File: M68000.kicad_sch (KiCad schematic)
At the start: 50 parts, among them J1 JTAG1, J2 USB_B, SW1 Util_SW, SW2 RESET_SW, SW3 STEP_SW, U1 MAX699, U2 XC9572, U3 MC68000FN, X1 ECS-2200B-080

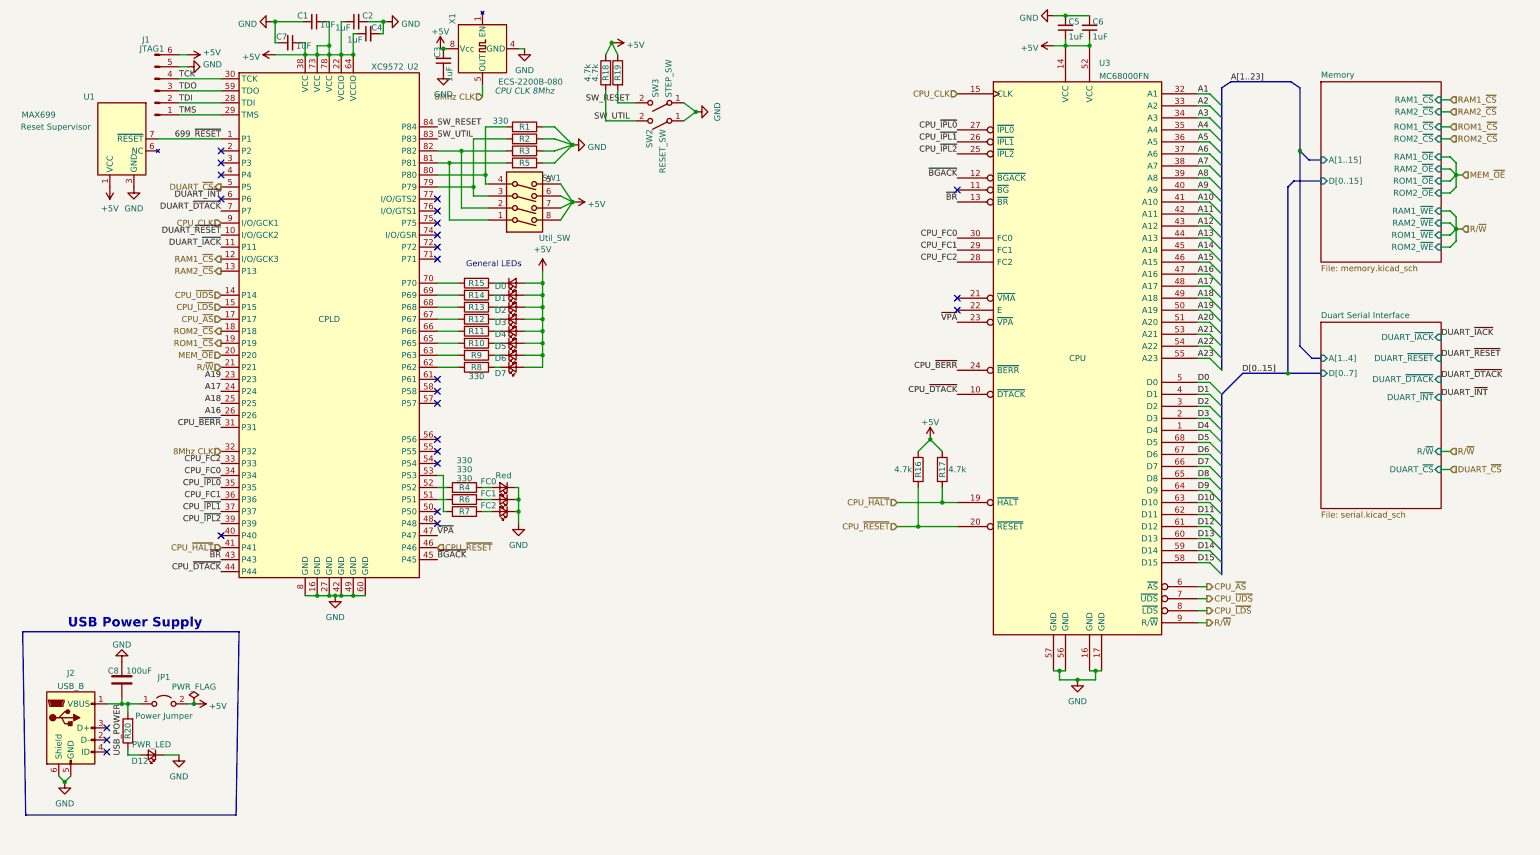
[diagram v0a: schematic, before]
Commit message: Submitted to JLCPCB
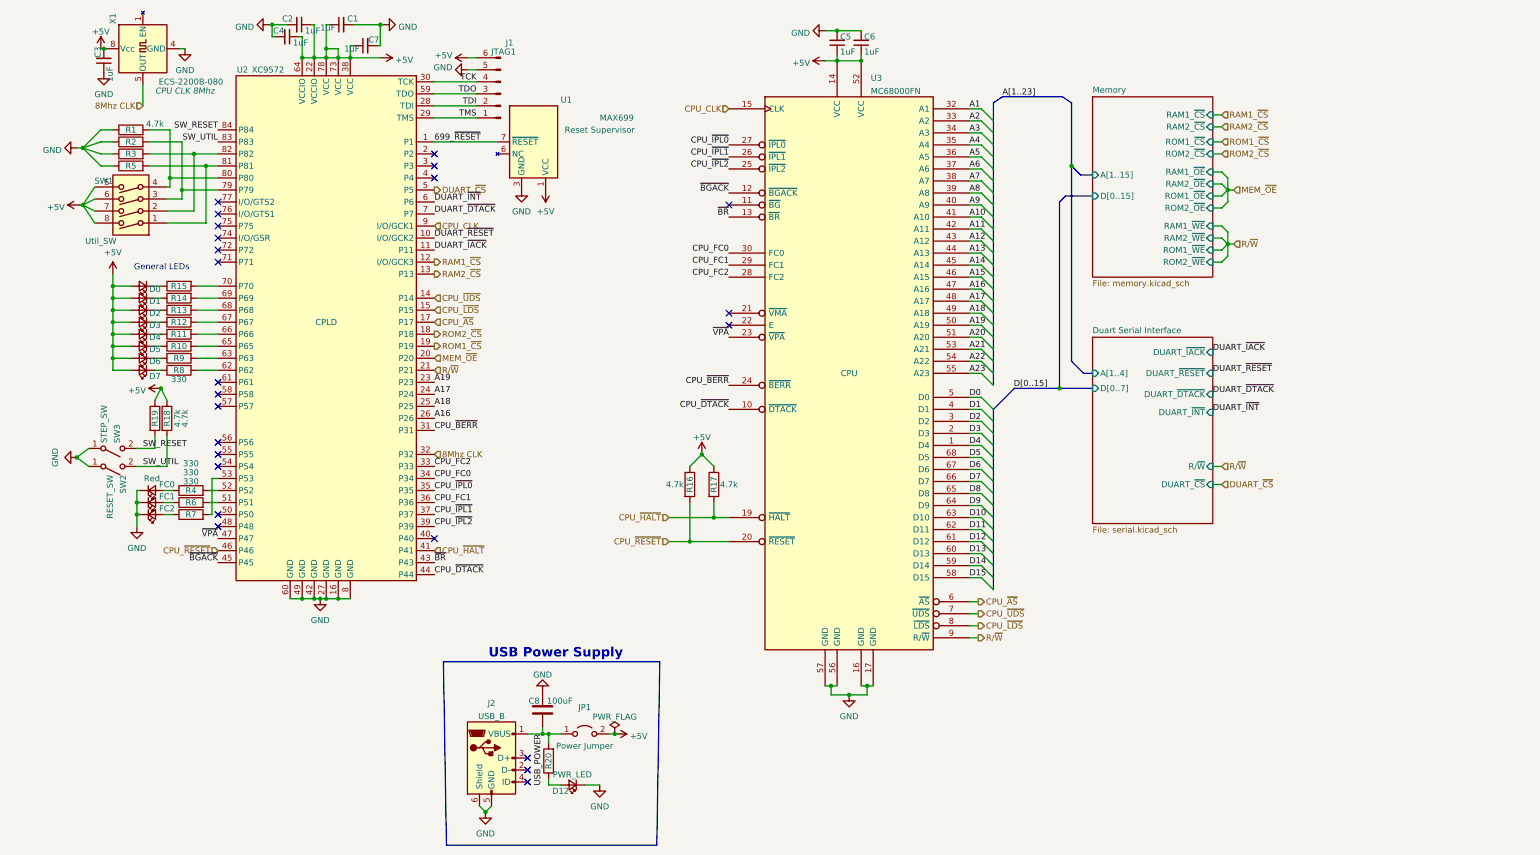
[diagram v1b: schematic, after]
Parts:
- R1, R2, R3, R5: value 330 -> 4.7k
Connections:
- no-connect marks 25 -> 24
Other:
- moved on the sheet: C1, C2, C3, C4, C5, C6, C7, C8, D0, D1, D12, D2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
